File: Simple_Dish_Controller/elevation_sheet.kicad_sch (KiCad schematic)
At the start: 20 parts, among them J2 1-Pin Terminal Block, J6 Conn_01x03_Pin, J7 RJ45 port shielded, RA, TH, J8 RJ45 port shielded, RA, TH, Q1 PZT2222A, Q2 PZT2222A, U2 74LS08, U3 74LS32, U4 NE555D

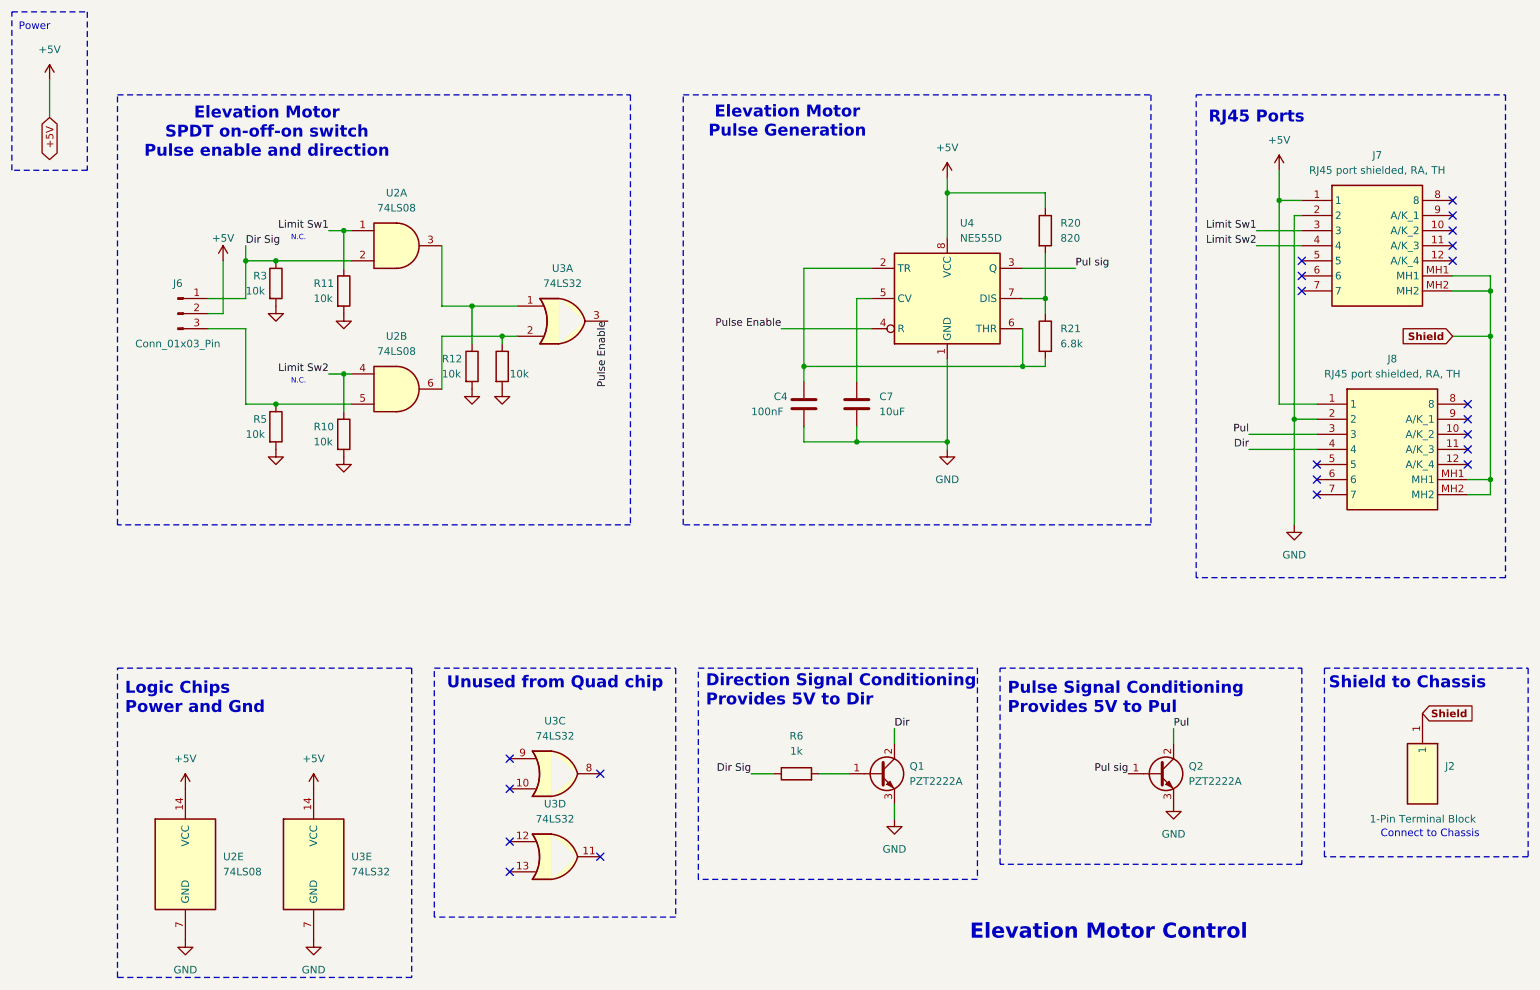
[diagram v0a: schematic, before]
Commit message: Latest update
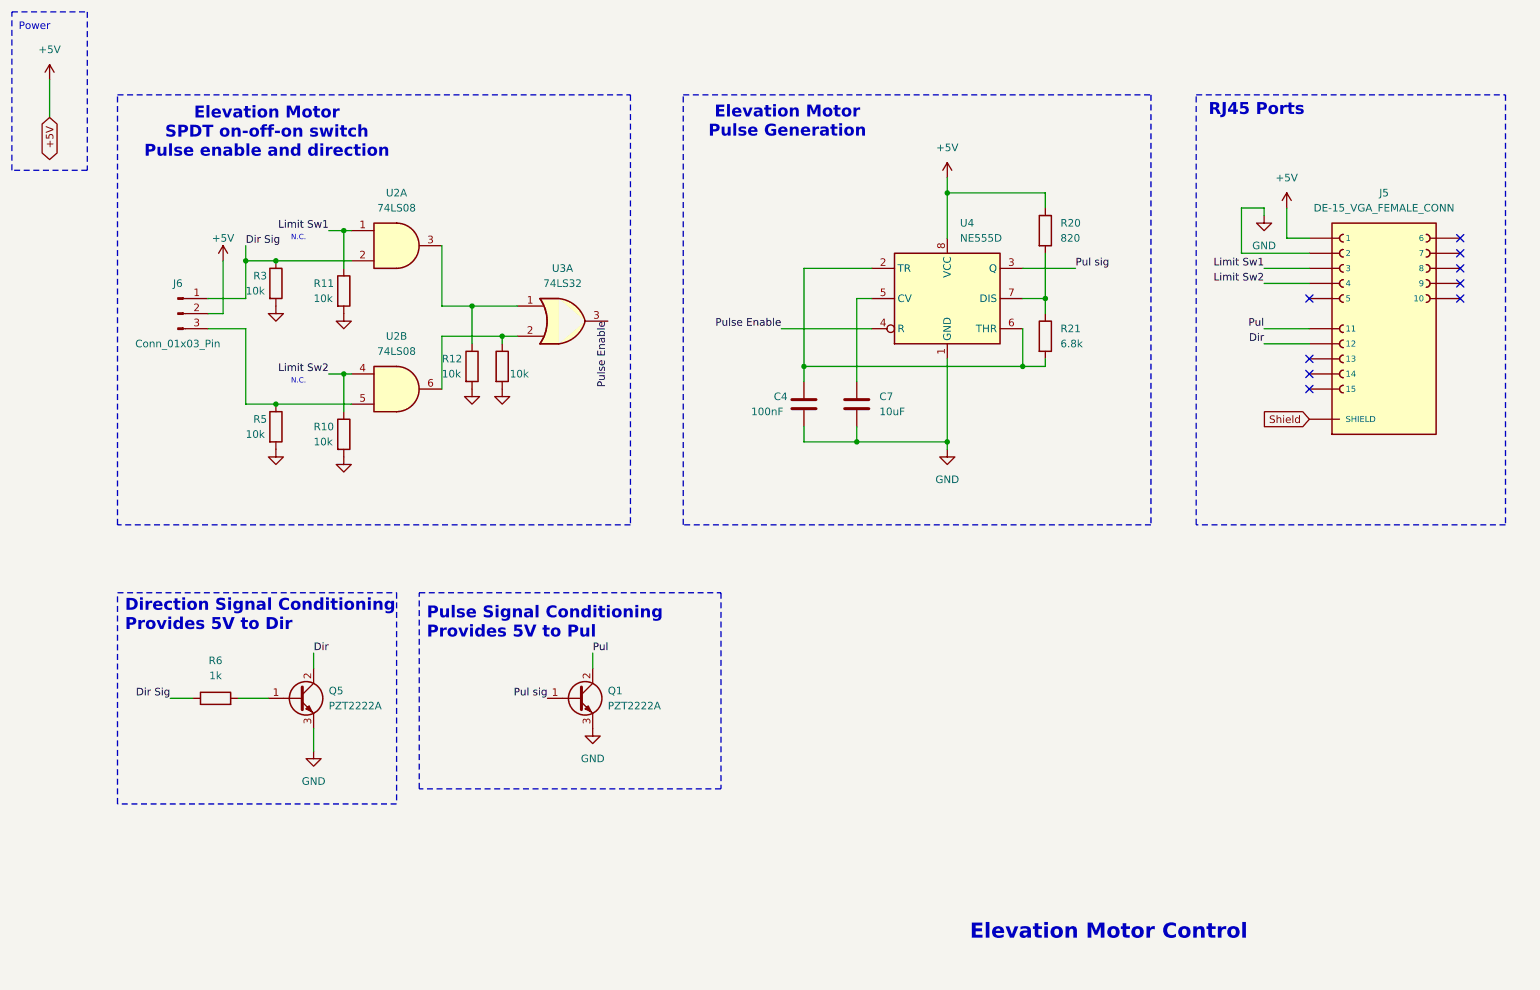
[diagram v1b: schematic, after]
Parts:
- removed J2: 1-Pin Terminal Block, 1-Pin Barrier Terminal Block:RHDR1W160P0X826_1X1_1020X1270X1270P, symbol 1-Pin Barrier Terminal Block:38700-6301
- removed J7, J8: RJ45 port shielded, RA, TH, DishController_footprints:RJ45 Port Shielded, Right Angle TH, symbol DishController_symbols:RJ45 port shielded, Right Angle TH
- removed Q1, Q2: PZT2222A, Package_TO_SOT_SMD:SOT-223-3_TabPin2, symbol Transistor_BJT:PZT2222A
- removed U2: 74LS08, 74LS08_SOIC:SOIC127P600X175-14N, symbol 74xx:74LS08
- removed U3: 74LS32, 74LS32_SOIC:SOIC127P600X175-14N, symbol 74xx:74LS32
- added J5: DE-15_VGA_FEMALE_CONN, DishFootprintsSupplier:DB15_VGA_FEMALE_CONN, symbol DishSymbolsSupplier:DE-15_VGA_FEMALE_CONN
- added Q1, Q5: PZT2222A, DishFootprints:SOT-223, symbol DishSymbols:PZT2222A
- added U2: 74LS08, DishFootprints:SOIC-14_3.9x8.7mm_P1.27mm, symbol DishSymbols:74LS08
- added U3: 74LS32, DishFootprints:SOIC-14_3.9x8.7mm_P1.27mm, symbol DishSymbols:74LS32
- R13: footprint Resistor_SMD:R_0805_2012Metric -> DishFootprints:R_0805
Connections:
- net +5V: now also J5.1
- net Dir: now also J5.12, Q5.2 (C)
- net Dir Sig: now also U2.2
- net GND: now also J5.2, Q1.3 (E), Q5.3 (E)
- net Limit Sw1: now also J5.3, U2.1
- net Limit Sw2: now also J5.4, U2.4
- net Pul: now also J5.11, Q1.2 (C)
- net Pul sig: now also Q1.1 (B)
- net Pulse Enable: now also U3.3
- net Shield: now also J5.SH1 (SHIELD), J5.SH2 (SHIELD)
- net at R13.1: now also U2.6, U3.2
- net at J6.3, R5.1: now also U2.5
- net at R6.2: now also Q5.1 (B)
- net at R12.1: now also U2.3, U3.1
- no-connect marks 22 -> 9
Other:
- note removed: "Connect to Chassis"
- note removed: "Logic Chips Power and Gnd"
- note removed: "Shield to Chassis"
- note removed: "Unused from Quad chip"
- moved on the sheet: R6

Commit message: Updates
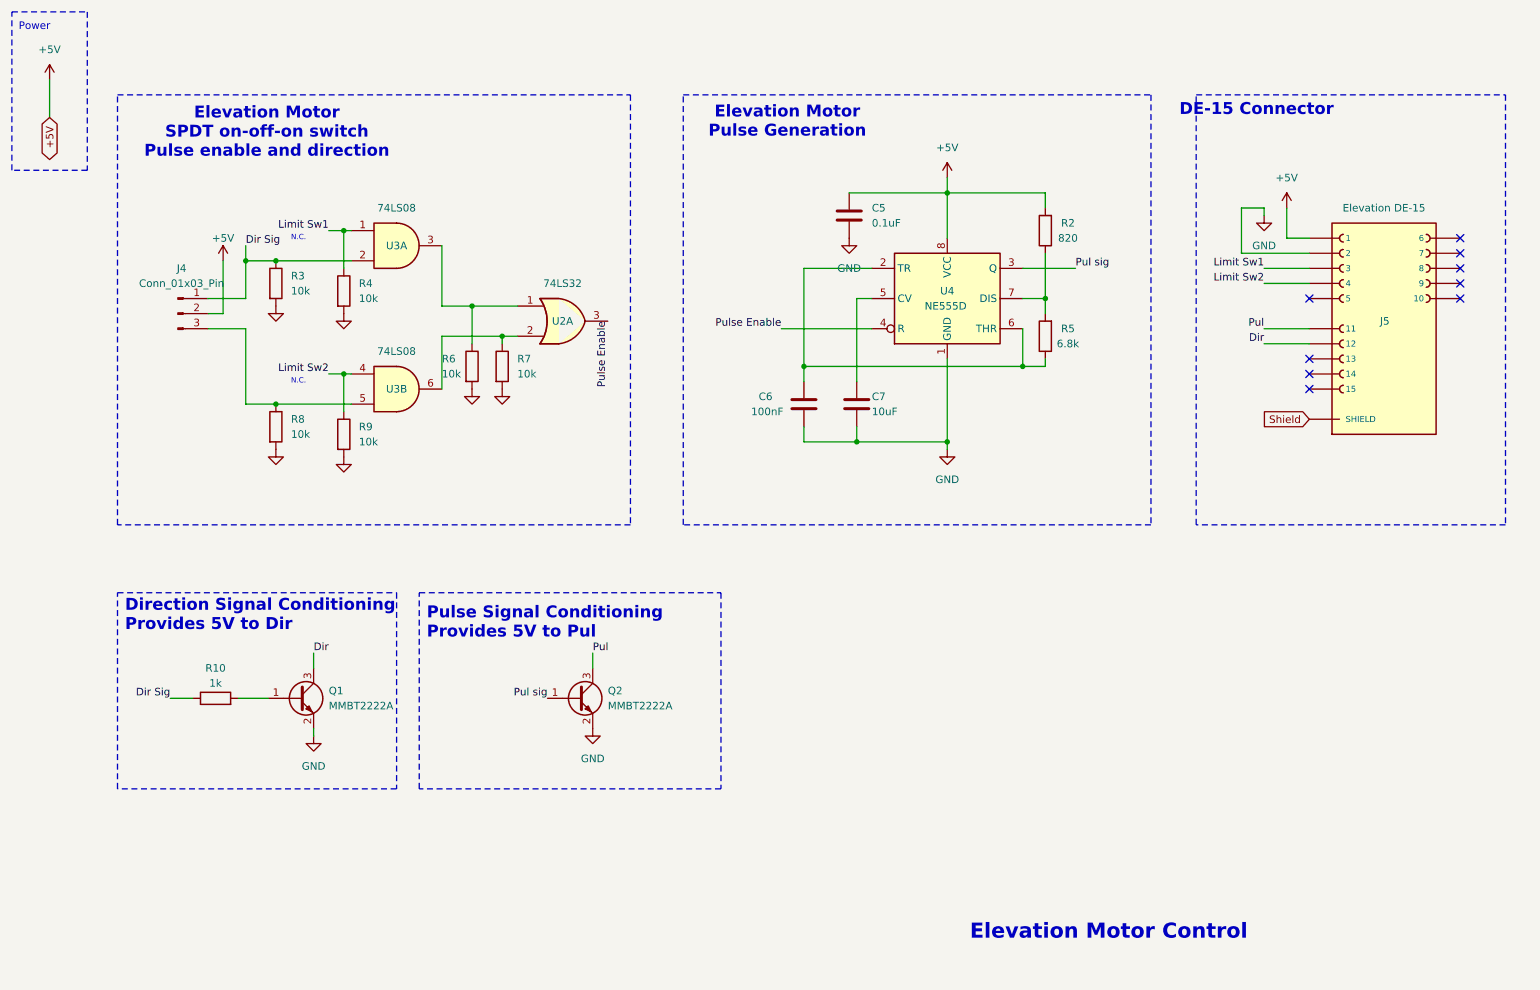
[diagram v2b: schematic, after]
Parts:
- removed C4: 100nF, DishFootprints:C_0805, symbol DishSymbols:CAP 100nF 0805
- removed C7: 10uF, DishFootprints:C_0805, symbol DishSymbols:CAP 10nF 0805
- removed J5: DE-15_VGA_FEMALE_CONN, DishFootprintsSupplier:DB15_VGA_FEMALE_CONN, symbol DishSymbolsSupplier:DE-15_VGA_FEMALE_CONN
- removed J6: Conn_01x03_Pin, DishFootprints:PinHeader_1x03_P2.54mm_Vertical, symbol DishSymbols:Conn_01x03_Pin
- removed Q1, Q5: PZT2222A, DishFootprints:SOT-223, symbol DishSymbols:PZT2222A
- removed R11, R12: 10k, Resistor_SMD:R_0805_2012Metric, symbol Device:R
- removed R13: 10k, DishFootprints:R_0805, symbol Device:R
- removed R20: 820, DishFootprints:R_0805, symbol DishSymbols:RES 820 0805
- removed R21: 6.8k, DishFootprints:R_0805, symbol DishSymbols:RES 6.8k 0805
- removed U2: 74LS08, DishFootprints:SOIC-14_3.9x8.7mm_P1.27mm, symbol DishSymbols:74LS08
- removed U3: 74LS32, DishFootprints:SOIC-14_3.9x8.7mm_P1.27mm, symbol DishSymbols:74LS32
- removed U4: NE555D, DishFootprints:SOIC-8_3.9x4.9mm_P1.27mm, symbol DishSymbols:NE555D
- added C5: 0.1uF, Capacitor_SMD:C_1206_3216Metric, symbol Device:C
- added C6: 100nF, Capacitor_SMD:C_1206_3216Metric, symbol Device:C
- added C7: 10uF, Capacitor_SMD:C_1206_3216Metric, symbol Device:C
- added J4: Conn_01x03_Pin, Connector_PinHeader_2.54mm:PinHeader_1x03_P2.54mm_Vertical, symbol Connector:Conn_01x03_Pin
- added J5: Elevation DE-15, DishFootprints:DE15_VGA_FEMALE_CONN, symbol DishSymbols:DE-15_VGA_FEMALE_CONN
- added Q1, Q2: MMBT2222A, Package_TO_SOT_SMD:SOT-23, symbol Transistor_BJT:MMBT2222A
- added R2: 820, Resistor_SMD:R_1206_3216Metric, symbol Device:R
- added R4, R7, R8, R9: 10k, Resistor_SMD:R_1206_3216Metric, symbol Device:R
- added U2: 74LS32, Package_SO:SOIC-14_3.9x8.7mm_P1.27mm, symbol 74xx:74LS32
- added U3: 74LS08, Package_SO:SOIC-14_3.9x8.7mm_P1.27mm, symbol 74xx:74LS08
- added U4: NE555D, Package_SO:SOIC-8_3.9x4.9mm_P1.27mm, symbol Timer:NE555D
- R10: value 10k -> 1k; footprint Resistor_SMD:R_0805_2012Metric -> Resistor_SMD:R_1206_3216Metric
- R3: footprint Resistor_SMD:R_0805_2012Metric -> Resistor_SMD:R_1206_3216Metric
- R5: value 10k -> 6.8k; footprint Resistor_SMD:R_0805_2012Metric -> Resistor_SMD:R_1206_3216Metric
- R6: value 1k -> 10k; footprint Resistor_SMD:R_0805_2012Metric -> Resistor_SMD:R_1206_3216Metric
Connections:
- net +5V: now also C5.1, J4.2 (Pin_2), J5.1, R2.2, U4.8 (VCC)
- net Dir: now also J5.12, Q1.3 (C)
- net Dir Sig: now also R10.1, J4.1 (Pin_1), U3.2; no longer R6.1
- net GND: now also R6.2, C5.2, C6.2, C7.2, J5.2, Q1.2 (E), Q2.2 (E), R4.2, R7.2, R8.2, R9.2, U4.1 (GND); no longer R10.2, R5.2
- net Limit Sw1: now also J5.3, R4.1, U3.1
- net Limit Sw2: now also J5.4, R9.1, U3.4; no longer R10.1
- net Pul: now also J5.11, Q2.3 (C)
- net Pul sig: now also Q2.1 (B), U4.3 (Q)
- net Pulse Enable: now also U2.3, U4.4 (R)
- net Shield: now also J5.SH1 (SHIELD), J5.SH2 (SHIELD)
- net at R5.1: now also C6.1, U4.2 (TR), U4.6 (THR)
- new net: J4.3 (Pin_3), R8.1, U3.5
- new net: R6.1, U2.1, U3.3
- new net: R7.1, U2.2, U3.6
- new net: R2.1, R5.2, U4.7 (DIS)
- new net: Q1.1 (B), R10.2
- new net: C7.1, U4.5 (CV)
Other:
- note added: "DE-15 Connector"
- note removed: "RJ45 Ports"
